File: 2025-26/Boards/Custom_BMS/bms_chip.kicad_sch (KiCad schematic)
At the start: 50 parts, among them J7 Conn_01x06_Pin, J8 15246140, Q1 BCX56-16,115, U1 BQ79616PAPRQ1

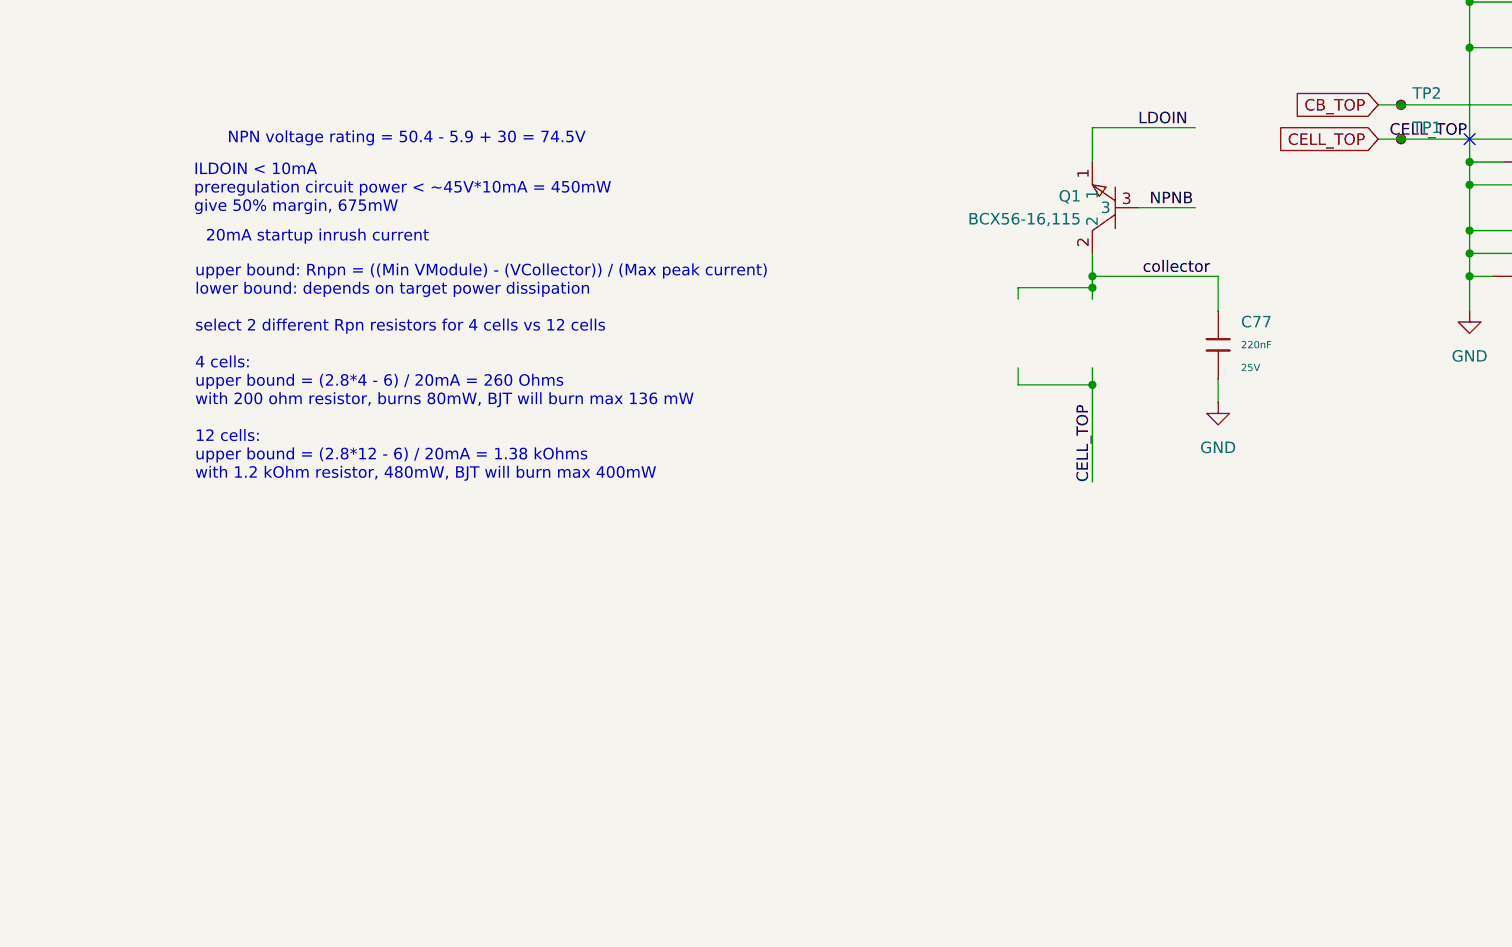
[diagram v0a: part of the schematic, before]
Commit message: fixed review items
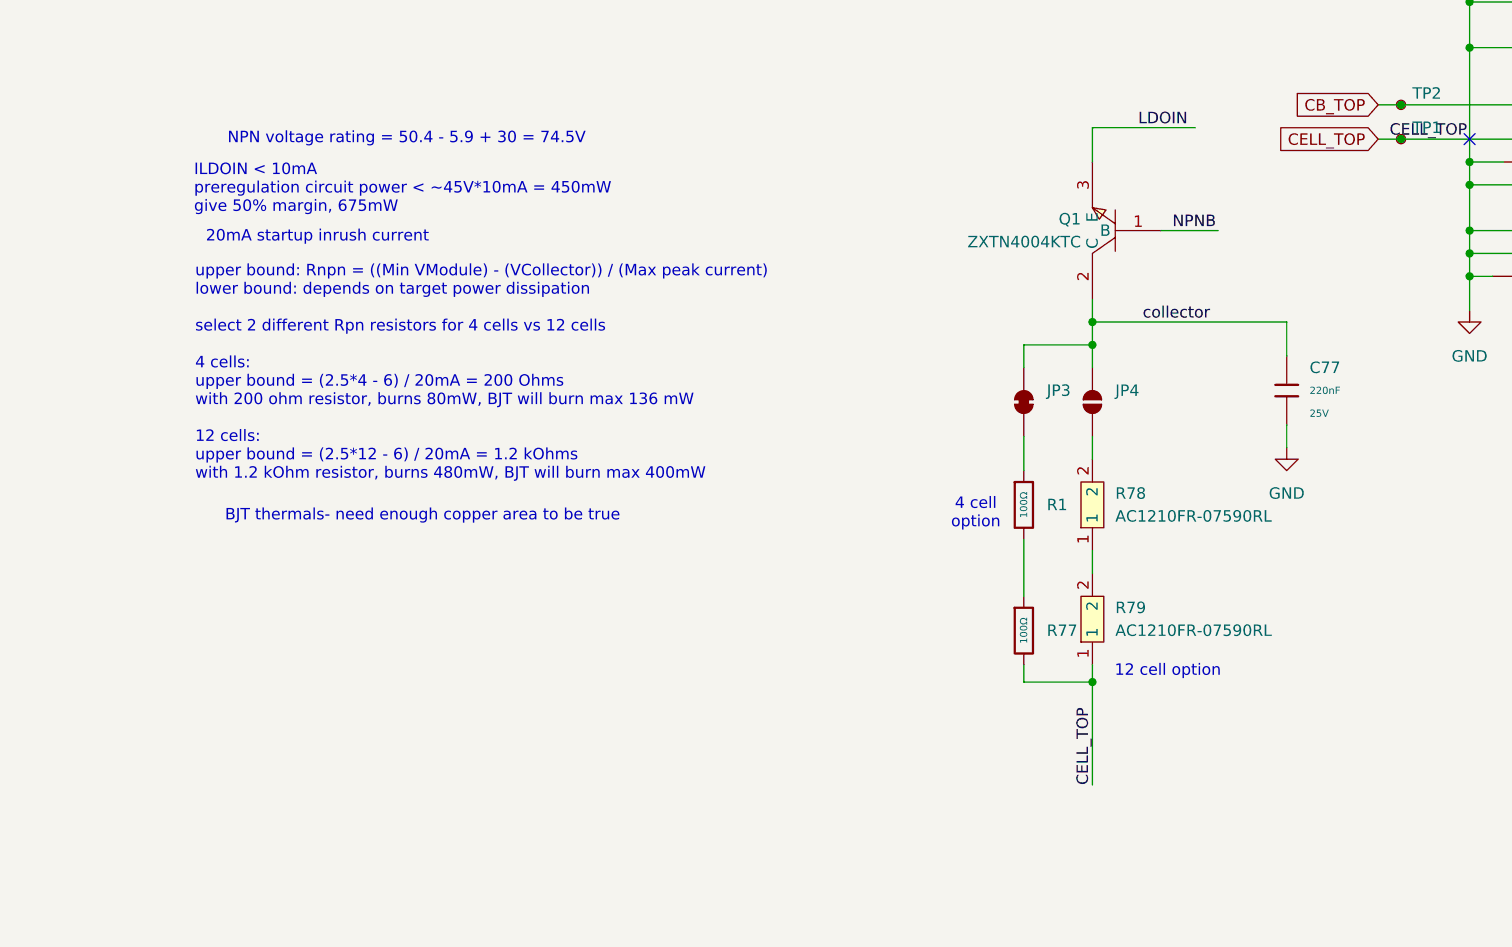
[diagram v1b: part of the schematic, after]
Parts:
- removed Q1: BCX56-16,115, easyeda2kicad:SOT-89-3_L4.5-W2.5-P1.50-LS4.1-TL-CW, symbol easyeda2kicad:BCX56-16,115
- added JP3: SolderJumper_2_Bridged, Jumper:SolderJumper-2_P1.3mm_Open_Pad1.0x1.5mm, symbol Jumper:SolderJumper_2_Bridged
- added JP4: SolderJumper_2_Open, Jumper:SolderJumper-2_P1.3mm_Open_Pad1.0x1.5mm, symbol Jumper:SolderJumper_2_Open
- added Q1: ZXTN4004KTC, easyeda2kicad:TO-252-2_L6.6-W6.1-P4.58-LS9.9-TL, symbol easyeda2kicad:ZXTN4004KTC
- added R1, R77: 100Ω, PCM_JLCPCB:R_0805, symbol PCM_JLCPCB-Resistors:0805,100Ω
- added R78, R79: AC1210FR-07590RL, easyeda2kicad:R1210, symbol easyeda2kicad:AC1210FR-07590RL
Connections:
- net CELL_TOP: now also R77.2, R79.1
- net LDOIN: now also Q1.3 (E)
- net NPNB: now also Q1.1 (B)
- net collector: now also JP3.2 (B), JP4.2 (B), Q1.2 (C)
- new net: R1.2, R77.1
- new net: JP4.1 (A), R78.2
- new net: JP3.1 (A), R1.1
- new net: R78.1, R79.2
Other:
- note added: "12 cell option"
- note added: "4 cell option"
- note added: "BJT thermals- need enough copper area to be true"
- note added: "upper bound: Rnpn = ((Min VModule) - (VCollector)) / (Max peak current) lower bound: depends on target power dissipation select 2 different Rpn resistors for 4 cells vs 12 cells 4 cells: upper bound = (2.5*4 - 6) / 20mA = 200 Ohms with 200 ohm resistor, burns 80mW, BJT will burn max 136 mW 12 cells: upper bound = (2.5*12 - 6) / 20mA = 1.2 kOhms with 1.2 kOhm resistor, burns 480mW, BJT will burn m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"
- note removed: "upper bound: Rnpn = ((Min VModule) - (VCollector)) / (Max peak current) lower bound: depends on target power dissipation select 2 different Rpn resistors for 4 cells vs 12 cells 4 cells: upper bound = (2.8*4 - 6) / 20mA = 260 Ohms with 200 ohm resistor, burns 80mW, BJT will burn max 136 mW 12 cells: upper bound = (2.8*12 - 6) / 20mA = 1.38 kOhms with 1.2 kOhm resistor, 480mW, BJT will burn max 40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"
- moved on the sheet: C77
